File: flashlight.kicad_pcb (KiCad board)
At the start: 2 copper layers, 45 x 120 mm, 25 parts, among them J1 USB_B_Micro, J2 Conn_01x03_Pin, Q1 HSS2333, Q2 HSS2333, SW1 SW_DIP_x01, U1 LP4054HB5F, U2 MT3608

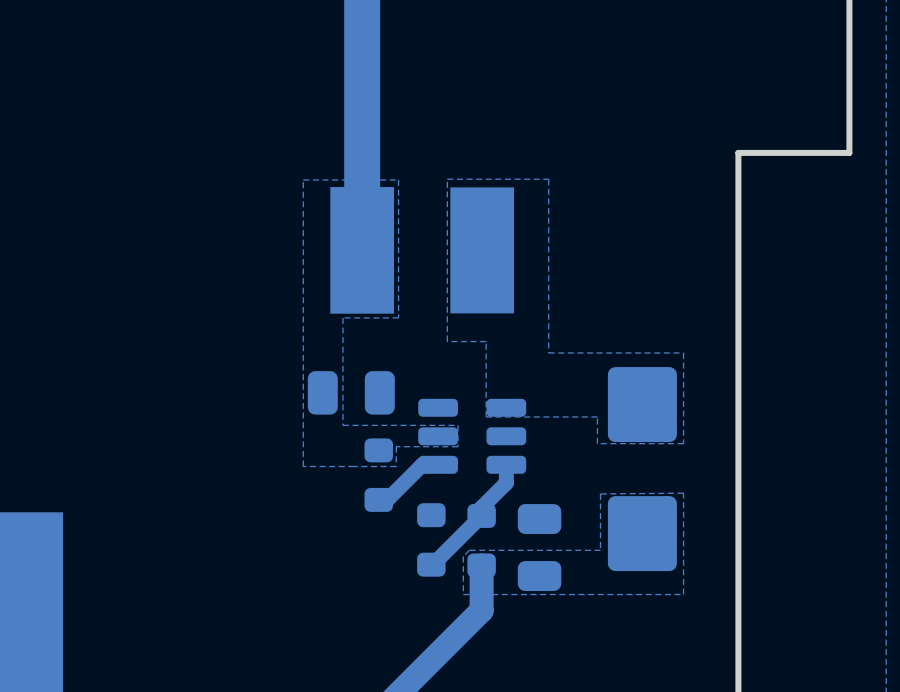
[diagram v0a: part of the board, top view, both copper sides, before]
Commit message: tight sot23-6
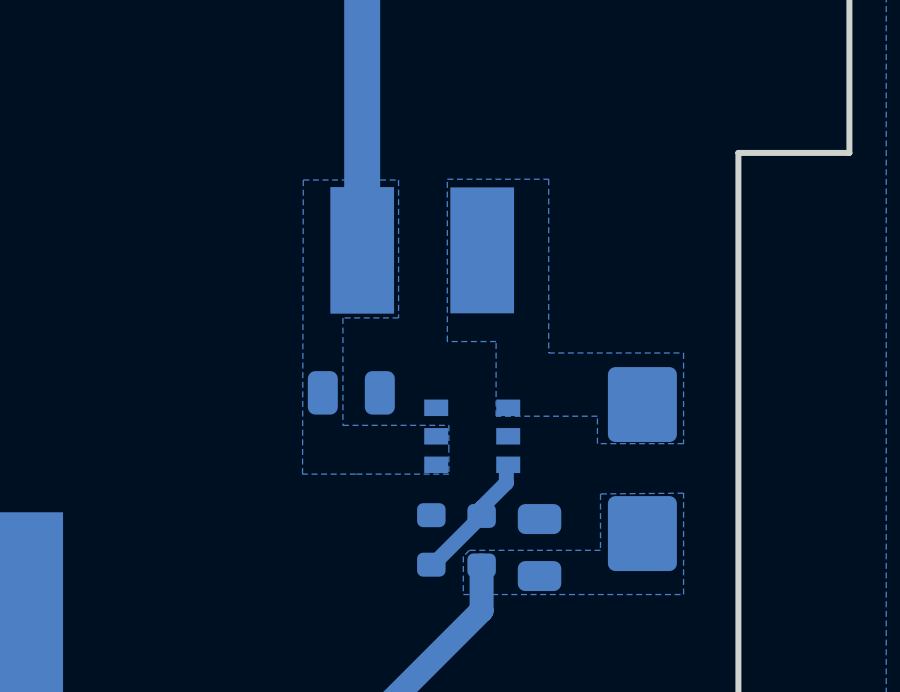
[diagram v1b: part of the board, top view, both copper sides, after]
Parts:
- removed R11: 10k, Resistor_SMD:R_0603_1608Metric
- U2: footprint Package_TO_SOT_SMD:SOT-23-6 -> SparkFun-Semiconductor-Standard:SOT23-6-Tight
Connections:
- C3 pad 1: Net-(U2-IN) -> Net-(U2-EN)
- L1 pad 1: Net-(U2-IN) -> Net-(U2-EN)
- SW1 pad 2: Net-(U2-IN) -> Net-(U2-EN)
- U2 pad 5: Net-(U2-IN) -> Net-(U2-EN)
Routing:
- net Net-(U2-IN): track 30.9 -> 0.00 mm
- net Net-(U2-EN): track 2.46 -> 30.9 mm
- added copper zone on B.Cu, net Net-(U2-EN)
- removed copper zone on B.Cu, net Net-(U2-IN)
